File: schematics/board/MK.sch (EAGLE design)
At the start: 19 parts

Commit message: ifdhv
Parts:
- added C2, C3, C4, C5: 100nF, rcl:C-EUC0603
- added R0, R11, R12, R13, R14, R15, R16, R17, R18, R19, R22, R23, R24, R25, R7, R8: 5k1, rcl:R-US_R0603
- added R20: (no value), rcl:R-US_R2512
- added R21: (no value), rcl:R-US_0207/15
- added U$0, U$10, U$11, U$12, U$5, U$7, U$8, U$9: VT93N1, KNPN-2023:VT93N1
- added U$13, U$15: 74HC595, CanCubeSat:74HC595
- added U$14: AD5593, UNKNOWN-2024:AD5593
- added U$16: INA219AID, CanCubeSat:INA219AID
- added U$17: IRF7905PBF, UNKNOWN-2024:IRF7905PBF
- added U$18, U$19, U$20: MOLEX-2-1.25, UNKNOWN-2024:MOLEX-2-1.25
- added U$3: BOARD_SHAPE, UNKNOWN-2024:BOARD_SHAPE
- added X1, X2: JST-2-2.5, UNKNOWN-2024:JST-2-2.5
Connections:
- new net BUS+: X1.1, X2.1
- new net FOTO0: U$20.2
- new net INA_SP+: R19.1, R20.1, R21.1
- new net LATCH: U$13.STCP, U$15.STCP
- new net MOSI: U$13.DS
- new net MOTOR1+: U$13.Q4, U$18.1
- new net MOTOR1-: U$13.Q5, U$18.2
- new net MOTOR2+: U$13.Q2, U$19.1
- new net MOTOR2-: U$13.Q3, U$19.2
- new net N$10: R14.2, U$11.1, U$14.IO6
- new net N$11: C2.1, U$14.VREF
- new net N$12: R15.2, U$12.1, U$14.IO7
- new net N$15: C5.2, R19.2, U$16.A0
- new net N$16: C3.1, C4.1, U$14.VDD, U$14.VDDL
- new net N$17: R16.1, U$14.AO
- new net N$18: C5.1, R18.2, U$16.A1
- new net N$19: R17.1, U$14.RESET
- new net N$20: U$17.D2, X1.2
- new net N$21: U$17.D1, X2.2
- new net N$22: R22.1, R23.2, U$17.G2
- new net N$23: R24.1, R25.2, U$17.G1
- new net N$35: U$13.Q7S, U$15.DS
- new net N$4: R0.2, U$0.1, U$14.IO0
- new net N$5: R8.2, U$14.IO2, U$7.1
- new net N$6: R7.2, U$14.IO1, U$5.1
- new net N$7: R11.2, U$14.IO3, U$8.1
- new net N$8: R12.2, U$14.IO4, U$9.1
- new net N$9: R13.2, U$10.1, U$14.IO5
- new net PERE1: R23.1, U$13.Q6
- new net PERE2: R25.1, U$13.Q7
- new net SCK: U$13.SHCP, U$15.SHCP
- new net SHIFT3: U$15.Q7S
- new net SP+: R18.1, R20.2
- new net SP-: R21.2
- net 3V3: now also R0.1, R11.1, R12.1, R13.1, R14.1, R15.1, R17.2, R7.1, R8.1, U$13.MR, U$13.VCC, U$15.MR, U$15.VCC, U$16.SCL
- net BUZZER: now also U$13.Q1
- net GND: now also C2.2, C3.2, C4.2, R16.2, R22.2, R24.2, U$0.2, U$10.2, U$11.2, U$12.2, U$13.GND, U$13.OE, U$14.GND, U$15.GND, U$15.OE, U$16.IN+, U$16.IN-, U$16.SDA, U$17.S1, U$17.S2, U$20.1, U$5.2, U$7.2, U$8.2, U$9.2
- net SCL: now also U$14.SCL, U$16.VS
- net SDA: now also U$14.SDA, U$16.GND

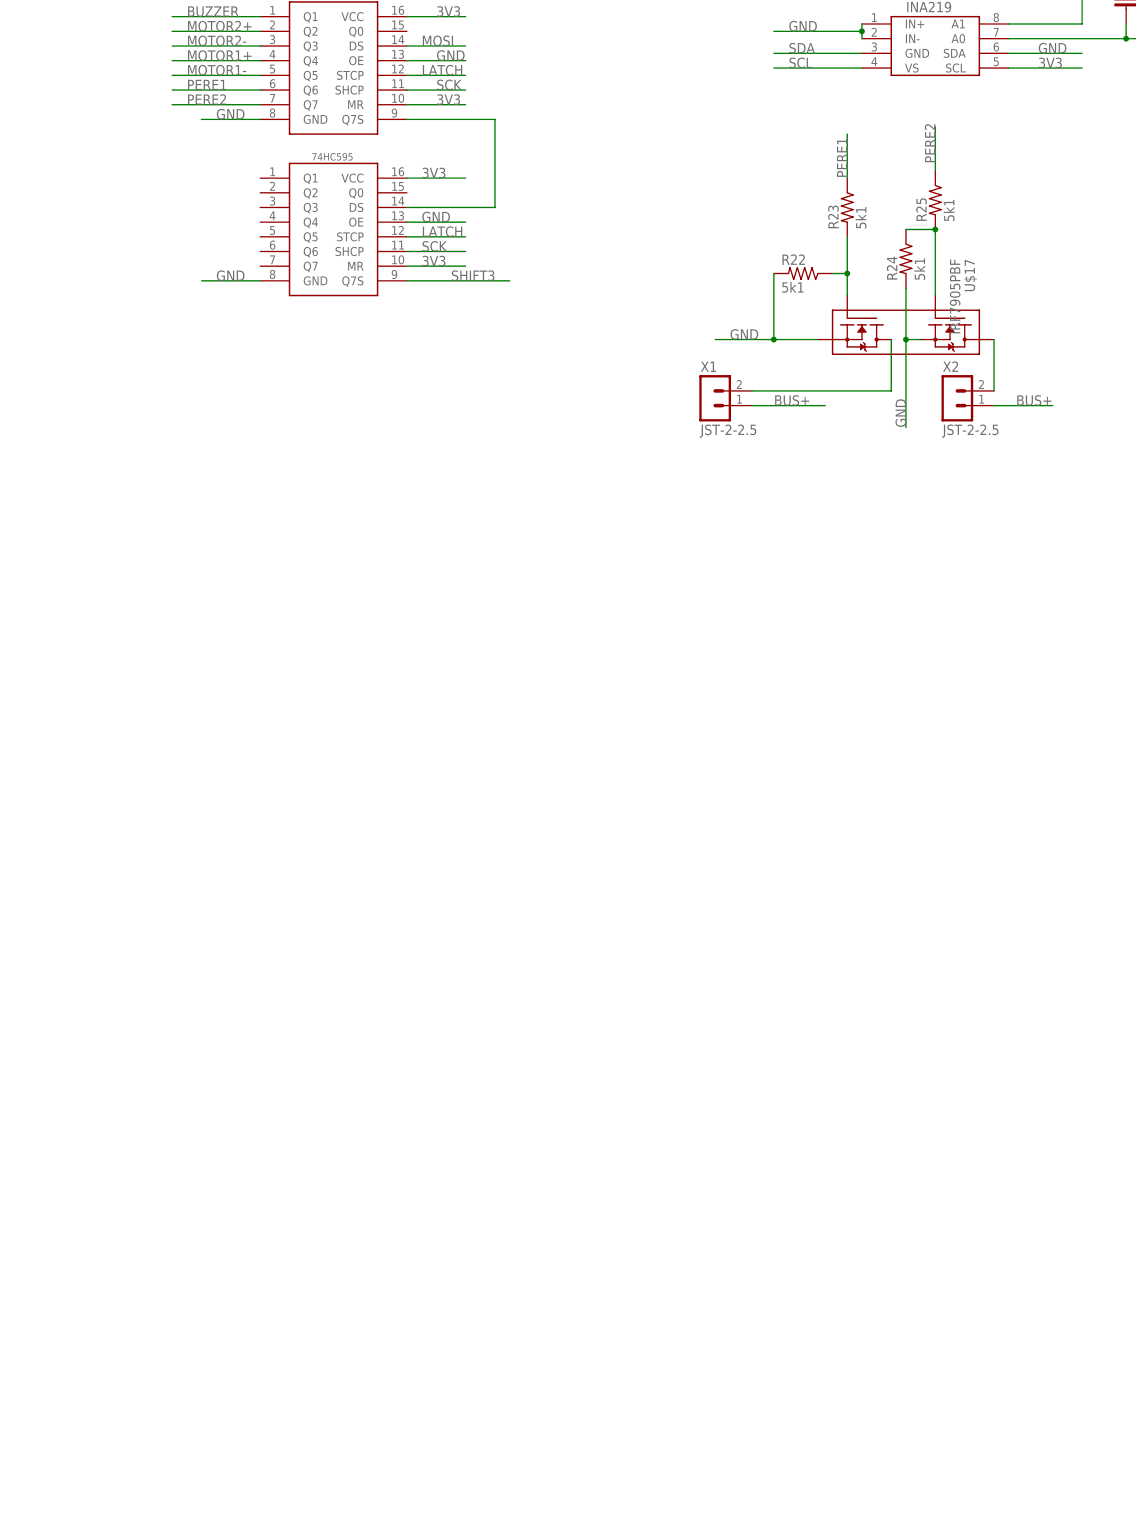
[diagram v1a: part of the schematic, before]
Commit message: пам пам тидам
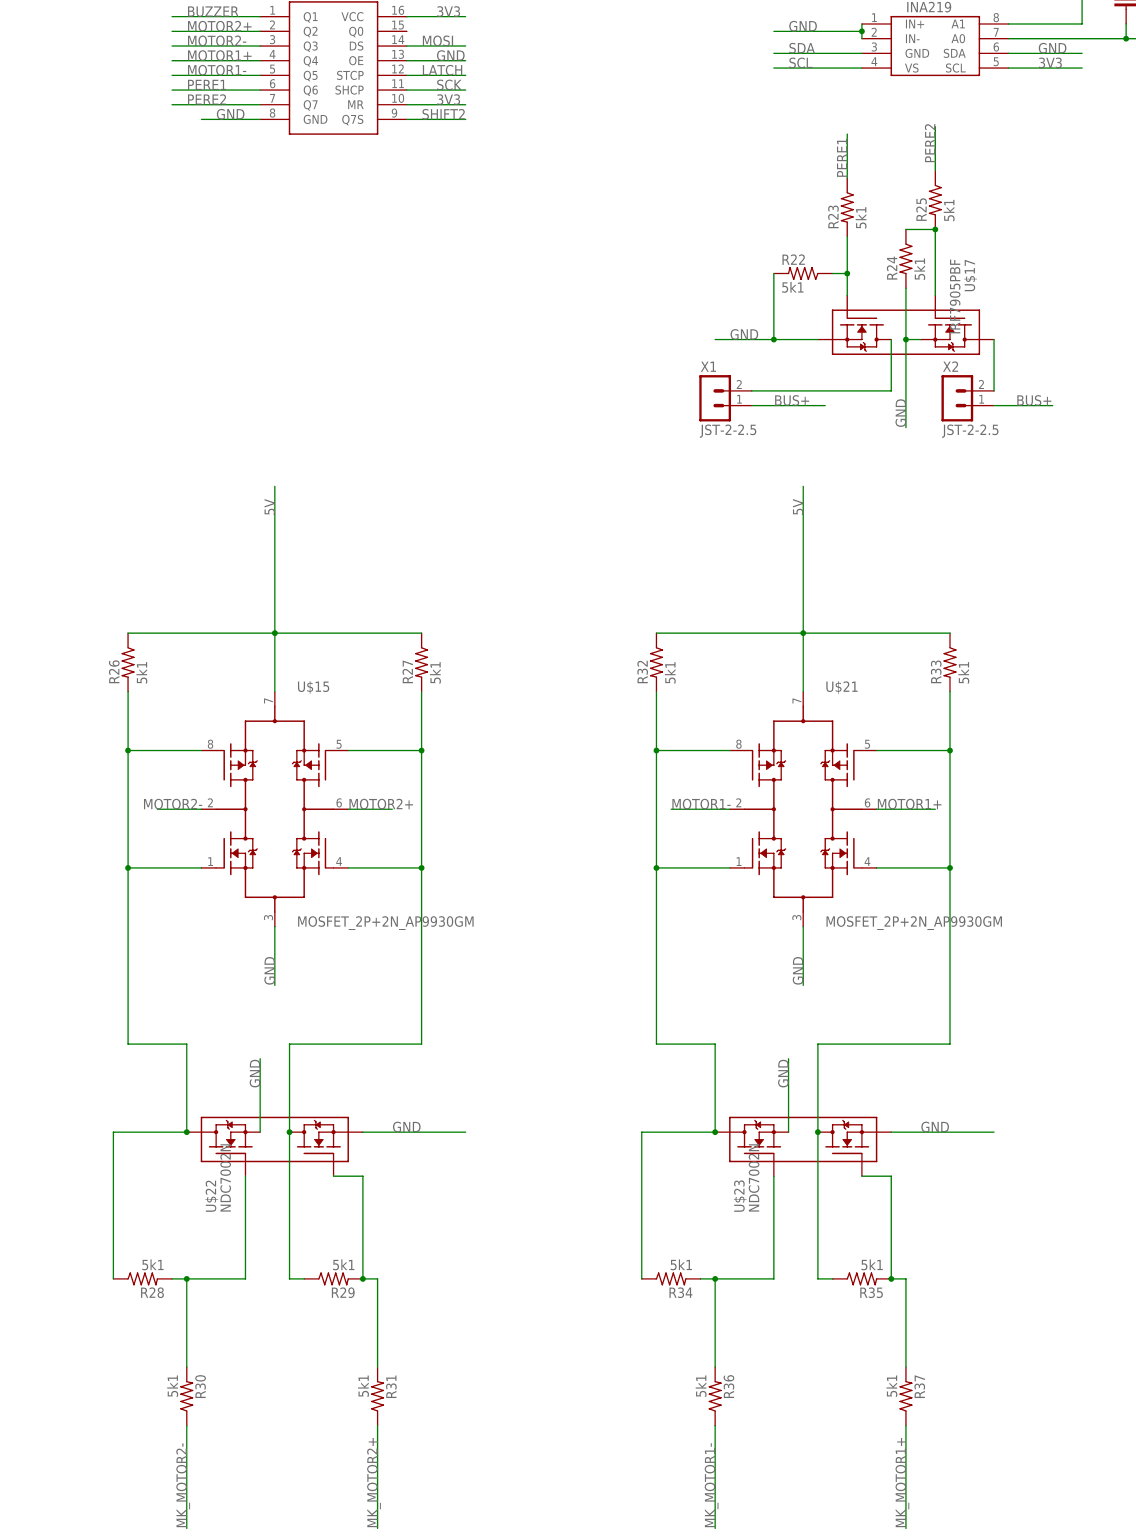
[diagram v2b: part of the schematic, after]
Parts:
- added R26, R27, R28, R29, R30, R31, R32, R33, R34, R35, R36, R37: 5k1, rcl:R-US_R0603
- added U$21: MOSFET_2P+2N_AP9930GM, UNKNOWN-2024:MOSFET_2P+2N_AP9930GM
- added U$22, U$23: NDC7002N, UNKNOWN-2024:NDC7002N
- U$15: value 74HC595 -> MOSFET_2P+2N_AP9930GM; device CanCubeSat:74HC595 -> UNKNOWN-2024:MOSFET_2P+2N_AP9930GM
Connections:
- removed net SHIFT3: U$15.Q7S
- new net MK_MOTOR1+: R37.1
- new net MK_MOTOR1-: R36.1
- new net MK_MOTOR2+: R31.1
- new net MK_MOTOR2-: R30.1
- new net N$24: R32.2, R34.1, U$21.N1G, U$21.P1G, U$23.D1
- new net N$25: R26.2, R28.1, U$15.N1G, U$15.P1G, U$22.D1
- new net N$26: R27.2, R29.1, U$15.N2G, U$15.P2G, U$22.D2
- new net N$27: R33.2, R35.1, U$21.N2G, U$21.P2G, U$23.D2
- new net N$28: R34.2, R36.2, U$23.G1
- new net N$29: R35.2, R37.2, U$23.G2
- new net N$32: R28.2, R30.2, U$22.G1
- new net SHIFT2: U$13.Q7S
- net 3V3: no longer U$15.MR, U$15.VCC
- net 5V: now also R26.1, R27.1, R32.1, R33.1, U$15.P1P2S, U$21.P1P2S
- net GND: now also U$15.N1N2S, U$21.N1N2S, U$22.S1, U$22.S2, U$23.S1, U$23.S2; no longer U$15.GND, U$15.OE
- net LATCH: no longer U$15.STCP
- net MOTOR1+: now also U$21.P2N2D
- net MOTOR1-: now also U$21.P1N1D
- net MOTOR2+: now also U$15.P2N2D
- net MOTOR2-: now also U$15.P1N1D
- net N$35: now also R29.2, R31.2, U$22.G2; no longer U$13.Q7S, U$15.DS
- net SCK: no longer U$15.SHCP

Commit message: Платки там
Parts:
- removed R15: 5k1, rcl:R-US_R0603
- removed U$10, U$11, U$12, U$5, U$7, U$8, U$9: VT93N1, KNPN-2023:VT93N1
- added JP1: (no value), pinhead:PINHD-1X10
- added JP2: (no value), pinhead:PINHD-1X16
- added R39, R40, R41, R42, R43, R44, R45, R46: 5k1, rcl:R-US_R0603
- R20: value (none) -> R05
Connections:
- net SD_CK renamed CK_SD
- removed net N$10: R14.2, U$11.1, U$14.IO6
- removed net N$12: R15.2, U$12.1, U$14.IO7
- removed net N$5: R8.2, U$14.IO2, U$7.1
- new net CO: R8.2, U$14.IO2
- new net CS_LIS: STM.PA10
- new net CS_LSM: STM.PA9
- new net H3: R12.2, U$14.IO4
- new net M0_RADIO: STM.PB1
- new net M1_RADIO: STM.PB10
- new net MICS: R13.2, U$14.IO5
- new net MISO_SENS: STM.PB4
- new net MOSI_SENS: STM.PB5
- new net N$34: R13.1, R45.2
- new net N$36: R12.1, R43.2
- new net N$37: R11.1, R41.2
- new net NO2: R11.2, U$14.IO3
- new net RX_GPS: STM.PA3
- new net RX_LIDAR: STM.PA12
- new net RX_RADIO: STM.PB3
- new net SCK_SENS: STM.PA5
- new net TX_GPS: STM.PA2
- new net TX_LIDAR: STM.PA11
- new net TX_RADIO: STM.PA15
- net 3V3: now also R40.1, R42.1, R44.1, R46.1; no longer R11.1, R12.1, R13.1, R14.1, R15.1, R8.1
- net 5V: now also R39.2, R8.1
- net ADC_FOTO: no longer STM.PA0
- net CE_RADIO: no longer STM.PC13
- net CS_RADIO: no longer STM.PC14
- net DIR_DRIVER: no longer STM.PA10
- net FOTO0: now also R7.2, U$14.IO1
- net GND: now also R14.1; no longer U$10.2, U$11.2, U$12.2, U$13.OE, U$5.2, U$7.2, U$8.2, U$9.2
- net IRQ_RADIO: no longer STM.PC15
- net MISO_RADIO: no longer STM.PA11
- net MISO_SR: no longer STM.PB4
- net MOSI_RADIO: no longer STM.PA1
- net MOSI_SR: no longer STM.PB5
- net N$6: now also R39.1, R40.2; no longer R7.2, U$14.IO1, U$5.1
- net N$7: now also R41.1, R42.2; no longer R11.2, U$14.IO3, U$8.1
- net N$8: now also R43.1, R44.2; no longer R12.2, U$14.IO4, U$9.1
- net N$9: now also R45.1, R46.2; no longer R13.2, U$10.1, U$14.IO5
- net OE_SR: now also R14.2, U$13.OE
- net RX1_BLE: no longer STM.PB3
- net RX2_GPS: no longer STM.PA3
- net SCK_RADIO: no longer STM.PB13
- net SCK_SR: no longer STM.PA5
- net STEP_DRIVER: no longer STM.PA9
- net SW_AMP: no longer STM.PA4
- net TX1_BLE: no longer STM.PA15
- net TX2_GPS: no longer STM.PA2
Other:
- moved on the sheet: BME280, BUZZER, C1, C2, C3, C4, C5, MICRO_SD, R0, R1, R10, R11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
